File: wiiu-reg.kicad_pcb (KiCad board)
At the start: 4 copper layers, 65.9 x 31.8 mm, 90 parts, among them IC1 SIC431CED-T1-GE3, IC2 SIC431CED-T1-GE3, IC3 NCP718ASNADJT1G, U1 AP62301Z6-7, U2 AP62301Z6-7, U3 AP62301Z6-7

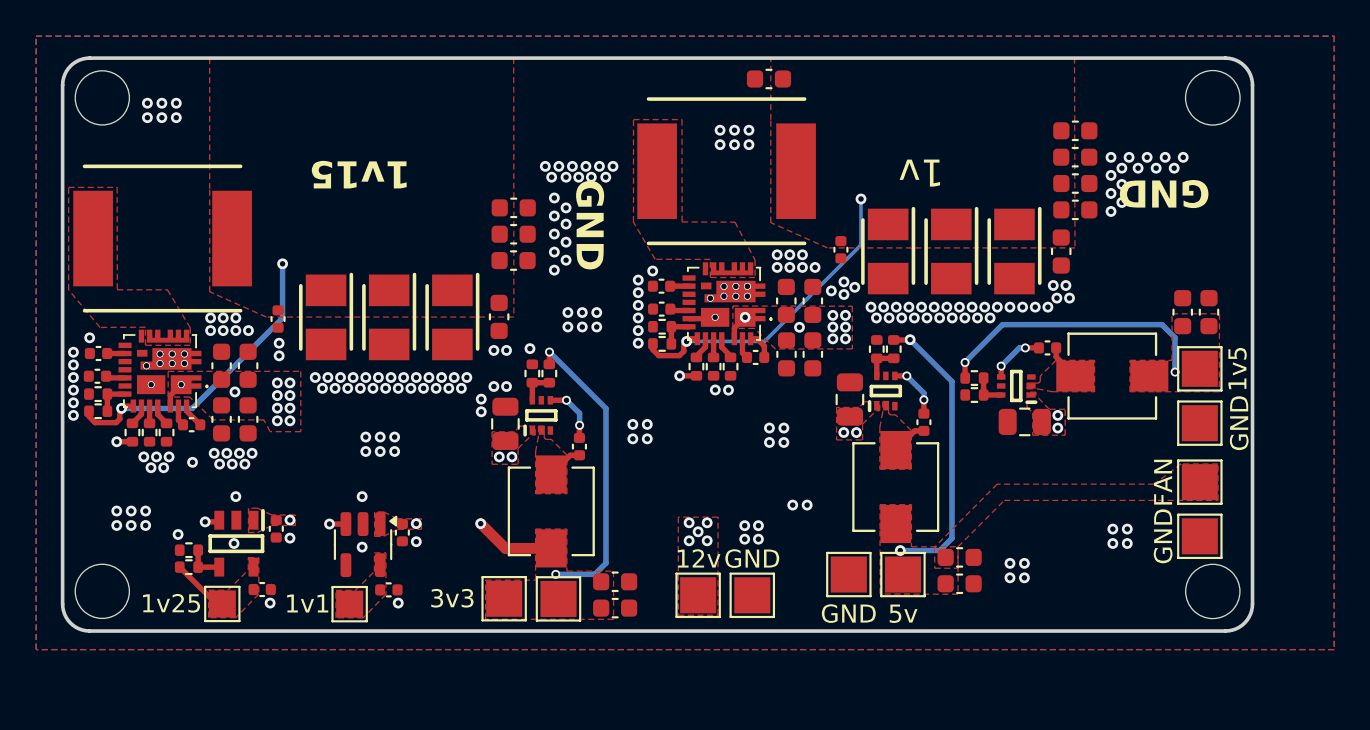
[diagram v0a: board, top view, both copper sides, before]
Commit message: Complete redesign
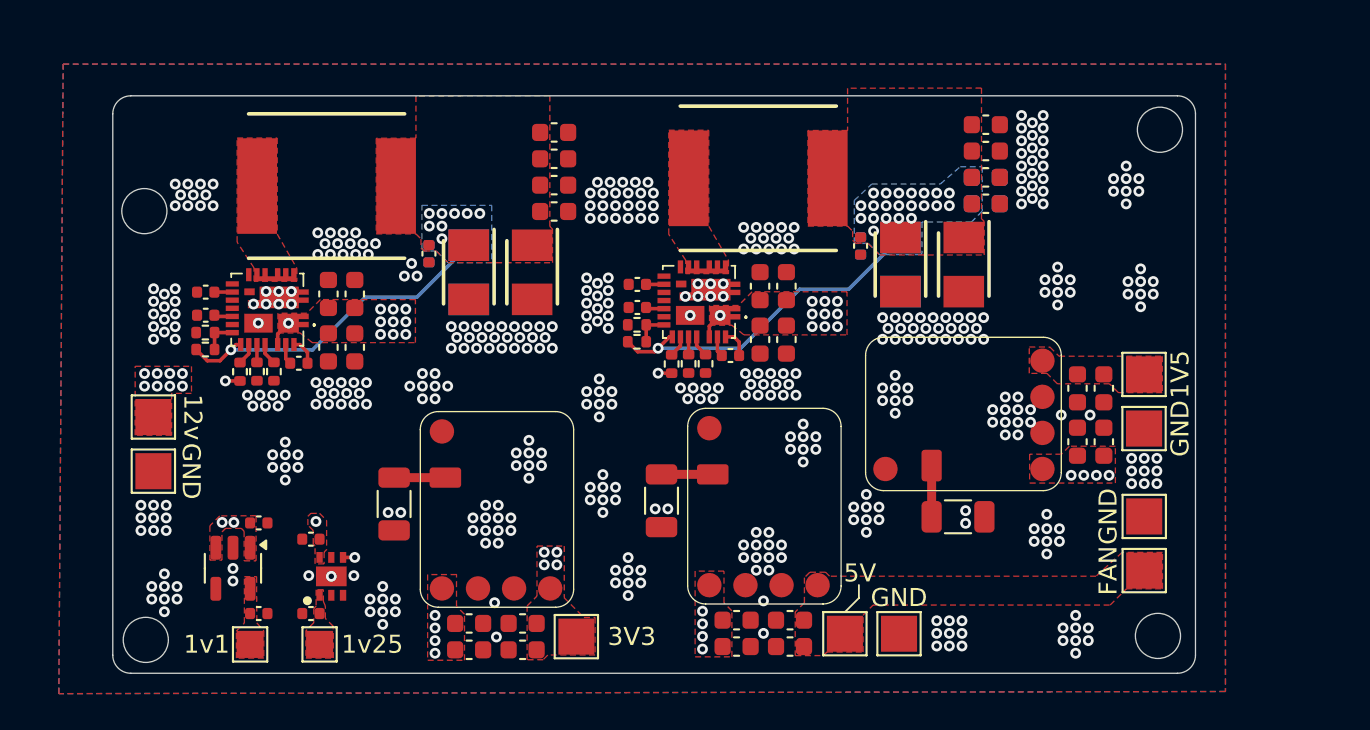
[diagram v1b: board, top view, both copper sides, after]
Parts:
- removed 1v5: 1v5, TestPoint:TestPoint_Pad_2.0x2.0mm
- removed 3v3, 3v31: 3v3, TestPoint:TestPoint_Pad_2.0x2.0mm
- removed 5v: 5v, TestPoint:TestPoint_Pad_2.0x2.0mm
- removed the GND at (140.2, 105.8)
- removed the GND at (165.0, 96.2)
- removed the GND at (145.6, 104.6)
- removed the GND at (165.0, 102.5)
- removed L3, L5: 3.3uH, wiiu-reg:INDM4847X300N
- removed L4: MPXV1D0840L1R0, wiiu-reg:MPXV1D0840L1R0
- removed R14: 510k, Resistor_SMD:R_0402_1005Metric
- removed R15: 8.66k, Resistor_SMD:R_0402_1005Metric
- removed R16, R17: 10k, Resistor_SMD:R_0402_1005Metric
- removed R18: 500, Resistor_SMD:R_0402_1005Metric
- added 1V5: 1v5, TestPoint:TestPoint_Pad_2.0x2.0mm, F.Cu at (161.9, 93.5)
- added 3V3: 3v3, TestPoint:TestPoint_Pad_2.0x2.0mm, F.Cu at (130.5, 108.1)
- added 5V: 5v, TestPoint:TestPoint_Pad_2.0x2.0mm, F.Cu at (145.3, 107.9)
- added C49: 1uF, Capacitor_SMD:C_0402_1005Metric, F.Cu at (112.9, 101.8)
- added C50: 1uF, Capacitor_SMD:C_0402_1005Metric, F.Cu at (112.9, 106.8)
- added GND: GND, TestPoint:TestPoint_Pad_2.0x2.0mm, F.Cu at (161.9, 101.4)
- added GND: GND, TestPoint:TestPoint_Pad_2.0x2.0mm, F.Cu at (107.0, 98.9)
- added GND: GND, TestPoint:TestPoint_Pad_2.0x2.0mm, F.Cu at (148.3, 107.9)
- added GND: GND, TestPoint:TestPoint_Pad_2.0x2.0mm, F.Cu at (161.9, 96.5)
- C1: value 100nF -> F930J107KBA; footprint Capacitor_SMD:C_0402_1005Metric -> wiiu-reg:F930J107KBA; moved to B.Cu
- C10, C11, C5: moved to B.Cu
- C16: value 10uF -> 0.1uF; footprint Capacitor_SMD:C_0805_2012Metric -> Capacitor_SMD:C_0402_1005Metric
- C17, C33: value 22uF -> 1uF; footprint Capacitor_SMD:C_0603_1608Metric -> Capacitor_SMD:C_0402_1005Metric
- C18, C34: value 22uF -> 2.2uF; footprint Capacitor_SMD:C_0603_1608Metric -> Capacitor_SMD:C_0402_1005Metric
- C19: value 0.1uF -> F930J107KBA; footprint Capacitor_SMD:C_0402_1005Metric -> wiiu-reg:F930J107KBA
- C20: value 1uF -> F930J107KBA; footprint Capacitor_SMD:C_0402_1005Metric -> wiiu-reg:F930J107KBA
- C21: value 2.2uF -> F930J107KBA; footprint Capacitor_SMD:C_0402_1005Metric -> wiiu-reg:F930J107KBA; moved to B.Cu
- C22: value 100nF -> 0.1uF
- C23: value 10uF -> 0.1uF; footprint Capacitor_SMD:C_0805_2012Metric -> Capacitor_SMD:C_0402_1005Metric; moved to B.Cu
- C26, C27, C28: value F930J107KBA -> 22uF; footprint wiiu-reg:F930J107KBA -> Capacitor_SMD:C_0603_1608Metric
- C29, C38: value 0.1uF -> 22uF; footprint Capacitor_SMD:C_0402_1005Metric -> Capacitor_SMD:C_0603_1608Metric
- C32: value 22uF -> 0.1uF; footprint Capacitor_SMD:C_0603_1608Metric -> Capacitor_SMD:C_0402_1005Metric
- C39, C45, C46: value 1uF -> 22uF; footprint Capacitor_SMD:C_0402_1005Metric -> Capacitor_SMD:C_0603_1608Metric
- C4: value F930J107KBA -> 0.1uF; footprint wiiu-reg:F930J107KBA -> Capacitor_SMD:C_0402_1005Metric
- C40: value 2.2uF -> 22uF; footprint Capacitor_SMD:C_0402_1005Metric -> Capacitor_SMD:C_0603_1608Metric
- C41: value 100nF -> 22uF; footprint Capacitor_SMD:C_0402_1005Metric -> Capacitor_SMD:C_0603_1608Metric
- C42: value 10uF -> 22uF; footprint Capacitor_SMD:C_0805_2012Metric -> Capacitor_SMD:C_0603_1608Metric
- IC3: value NCP718ASNADJT1G -> TPS7A26125DRVR; footprint wiiu-reg:NCP718ASNADJT1G -> wiiu-reg:TPS7A26125DRVR
- L2: value 3.3uH -> MPXV1D0840L1R0; footprint wiiu-reg:INDM4847X300N -> wiiu-reg:MPXV1D0840L1R0
- R10, R4, R5: value 10k -> 510k
- R11: value 100k -> 7.5k; footprint Resistor_SMD:R_0402_1005Metric -> Resistor_SMD:R_1206_3216Metric
- R12: value 12k -> 2.61k; footprint Resistor_SMD:R_0402_1005Metric -> Resistor_SMD:R_1206_3216Metric
- R13: value 510k -> 1.58k; footprint Resistor_SMD:R_0402_1005Metric -> Resistor_SMD:R_1206_3216Metric
- R2: value 52.3k -> 100k
- R3: value 100k -> 10k
- R6: value 510k -> 11k
- R7: value 510k -> 100k
- R8: value 31.6k -> 12k
- R9: value 11k -> 510k
- U1, U2, U3: value AP62301Z6-7 -> ~; footprint wiiu-reg:AP62301Z6-7 -> wiiu-reg:Reggie
- moved C38 50.6 mm to (159.7, 94.3), turned to -90 degrees
- moved C36 49.1 mm to (159.7, 97.3)
- moved C35 47.4 mm to (158.2, 97.3), turned to 90 degrees
- moved R11 46.0 mm to (151.6, 101.4), turned to 0 degrees
- moved C37 46.0 mm to (158.2, 94.3), turned to -90 degrees
- moved L2 35.7 mm to (116.6, 83.1), turned to 0 degrees
- moved C41 32.9 mm to (127.5, 107.3), turned to 180 degrees
- moved 12v 31.8 mm to (107.0, 95.9), turned to 180 degrees
- moved C43 31.3 mm to (139.3, 107.2), turned to 0 degrees
- moved C44 30.9 mm to (139.3, 108.6), turned to 0 degrees
- moved C42 30.6 mm to (127.5, 108.8), turned to 180 degrees
- moved C46 29.4 mm to (142.3, 108.6), turned to 180 degrees
- moved R6 29.1 mm to (109.9, 92.2), turned to 0 degrees
- moved C45 28.9 mm to (142.3, 107.2), turned to 180 degrees
- moved R13 27.7 mm to (135.2, 100.5)
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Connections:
- net 1v SW renamed Net-(IC1-SW_1)
- C1 pad 1: Net-(U1-BST) -> +1V0
- C1 pad 2: Net-(U1-SW) -> GND
- C16 pad 1: GND -> Net-(IC1-BOOT)
- C16 pad 2: VIN -> Net-(IC1-PHASE)
- C17 pad 1: +5V -> Net-(IC1-VDD)
- C18 pad 1: +5V -> Net-(IC1-VDRV)
- C19 pad 1: Net-(IC1-BOOT) -> +1V15
- C19 pad 2: Net-(IC1-PHASE) -> GND
- C20 pad 1: Net-(IC1-VDD) -> +1V15
- C21 pad 1: Net-(IC1-VDRV) -> +1V15
- C22 pad 1: Net-(U2-BST) -> +1V15
- C22 pad 2: Net-(U2-SW) -> GND
- C23 pad 1: GND -> +1V15
- C23 pad 2: VIN -> GND
- C24 pad 1: +3V3 -> +1V15
- C25 pad 1: +3V3 -> +1V15
- C28 pad 1: +1V15 -> VIN
- C29 pad 1: +1V15 -> VIN
- C30 pad 1: +1V15 -> VIN
- C31 pad 1: +1V15 -> VIN
- C32 pad 1: +1V15 -> Net-(IC2-BOOT)
- C32 pad 2: GND -> Net-(IC2-PHASE)
- C33 pad 1: +1V15 -> Net-(IC2-VDD)
- C34 pad 1: VIN -> Net-(IC2-VDRV)
- C37 pad 1: VIN -> +1V5
- C38 pad 1: Net-(IC2-BOOT) -> +1V5
- C38 pad 2: Net-(IC2-PHASE) -> GND
- C39 pad 1: Net-(IC2-VDD) -> VIN
- C40 pad 1: Net-(IC2-VDRV) -> VIN
- C41 pad 1: Net-(U3-BST) -> +3V3
- C41 pad 2: Net-(U3-SW) -> GND
- C42 pad 1: GND -> +3V3
- C42 pad 2: VIN -> GND
- C43 pad 1: +1V5 -> VIN
- C44 pad 1: +1V5 -> VIN
- C45 pad 1: +3V3 -> +5V
- C46 pad 1: +1V25 -> +5V
- C47 pad 1: +3V3 -> +1V25
- C48 pad 1: +1V1 -> +3V3
- IC2 pad 30: 1v15 SW -> Net-(IC2-SW_1)
- IC2 pad 31: 1v15 SW -> Net-(IC2-SW_1)
- IC2 pad 32: 1v15 SW -> Net-(IC2-SW_1)
- IC2 pad 33: 1v15 SW -> Net-(IC2-SW_1)
- IC2 pad 5: 1v15 SW -> Net-(IC2-SW_1)
- IC2 pad 6: 1v15 SW -> Net-(IC2-SW_1)
- IC2 pad 7: 1v15 SW -> Net-(IC2-SW_1)
- IC2 pad 8: 1v15 SW -> Net-(IC2-SW_1)
- IC2 pad 9: 1v15 SW -> Net-(IC2-SW_1)
- IC3 pad 1: +3V3 -> +1V25
- IC3 pad 3: +3V3 -> GND
- IC3 pad 4: Net-(IC3-NC/ADJ) -> +3V3
- IC3 pad 5: +1V25 -> GND
- L2 pad 1: Net-(U1-SW) -> Net-(IC2-SW_1)
- L2 pad 2: +5V -> +1V15
- R10 pad 1: Net-(U2-FB) -> Net-(IC2-MODE2)
- R11 pad 1: VIN -> Net-(U1-FB)
- R11 pad 2: Net-(IC2-EN) -> GND
- R12 pad 1: Net-(IC2-FB) -> Net-(U2-FB)
- R13 pad 1: Net-(IC2-MODE1) -> Net-(U3-FB)
- R2 pad 1: +5V -> VIN
- R2 pad 2: Net-(U1-FB) -> Net-(IC1-EN)
- R3 pad 1: VIN -> Net-(IC1-FB)
- R3 pad 2: Net-(IC1-EN) -> GND
- R4 pad 1: Net-(IC1-FB) -> Net-(IC1-MODE1)
- R5 pad 1: Net-(U1-FB) -> Net-(IC1-MODE2)
- R6 pad 1: Net-(IC1-MODE1) -> +1V15
- R6 pad 2: GND -> Net-(IC2-FB)
- R7 pad 1: Net-(IC1-MODE2) -> VIN
- R7 pad 2: GND -> Net-(IC2-EN)
- R8 pad 1: +3V3 -> Net-(IC2-FB)
- R8 pad 2: Net-(U2-FB) -> GND
- R9 pad 1: +1V15 -> Net-(IC2-MODE1)
- R9 pad 2: Net-(IC2-FB) -> GND
- U1 pad 2: Net-(U1-SW) -> +1V5
- U1 pad 4: Net-(U1-BST) -> Net-(U1-FB)
- U2 pad 2: Net-(U2-SW) -> +3V3
- U2 pad 4: Net-(U2-BST) -> Net-(U2-FB)
- U3 pad 2: Net-(U3-SW) -> +5V
- U3 pad 4: Net-(U3-BST) -> Net-(U3-FB)
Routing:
- net +3V3: track 22.9 -> 0.65 mm, vias 7 -> 8
- net +5V: track 16.0 -> 0.00 mm, vias 2 -> 0
- net +1V5: track 15.6 -> 0.00 mm, vias 2 -> 0
- net Net-(U2-BST): track 3.29 -> 0.00 mm, vias 2 -> 0
- net +1V25: track 3.20 -> 0.00 mm
- net Net-(U1-BST): track 3.14 -> 0.00 mm, vias 2 -> 0
- net Net-(U3-BST): track 2.99 -> 0.00 mm, vias 2 -> 0
- net Net-(IC3-NC/ADJ): track 2.11 -> 0.00 mm
- net Net-(U2-SW): track 2.03 -> 0.00 mm
- net Net-(U3-SW): track 2.00 -> 0.00 mm
- net Net-(U1-SW): track 2.00 -> 0.00 mm
- net GND: track 1.59 -> 0.00 mm, vias 221 -> 434
- net +1V15: track 17.6 -> 18.7 mm, vias 2 -> 9
- net +1V0: track 18.0 -> 19.0 mm, vias 2 -> 22
- net Net-(U1-FB): track 1.91 -> 2.84 mm
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- added copper zone on B.Cu, net +1V0
- added copper zone on B.Cu, net +1V15
- added copper zone on In1.Cu, net +3V3
- added copper zone on In2.Cu, net GND
- added copper zone on F.Cu, net Net-(IC2-SW_1)
- added copper zone on In1.Cu, net VIN
- removed copper zone on In2.Cu, net +3V3
- removed copper zone on F.Cu, net 1v15 SW
- removed copper zone on In1.Cu, net GND
- removed copper zone on F.Cu, net Net-(U1-SW)
- removed copper zone on F.Cu, net Net-(U2-SW)
- removed copper zone on F.Cu, net Net-(U3-SW)
- removed copper zone on In2.Cu, net VIN
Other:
- board size 65.9 x 31.8 mm -> 60 x 32 mm
- board text removed: "PiiSU Lazr 2025 Name by pbanj"
